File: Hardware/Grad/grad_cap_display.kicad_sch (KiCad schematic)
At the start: 11 parts, among them J101 Conn_01x06, J102 Conn_01x06, J103 Conn_01x06, J104 Conn_01x06, J105 Conn_01x06, J106 Conn_01x06, J107 Conn_01x06, J108 Conn_01x06, J109 Conn_01x06

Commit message: Schematic feels done now
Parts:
- J101, J102, J103, J104, J105, J106, J107, J108, J109: value Conn_01x06 -> 6-Pos 2.54mm Header; footprint (none) -> Connector_PinHeader_2.54mm:PinHeader_1x06_P2.54mm_Vertical
- R101, R102: footprint (none) -> New_Library:Worthington_R_0402
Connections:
- net RS485_B renamed FRAME_SYNC
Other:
- added sheet SAMD21 (SAMD21.kicad_sch)
- sheet ESP32 1 ports: added BACKLIGHT_PWM_IN, FRAME_SYNC_IN, SPI_CS_µSD, SPI_MISO_µSD, SPI_MOSI_µSD, SPI_SCK_µSD; removed FRAME_SYNC
- sheet ESP32 2 ports: added BACKLIGHT_PWM_IN, FRAME_SYNC_IN, SPI_CS_µSD, SPI_MISO_µSD, SPI_MOSI_µSD, SPI_SCK_µSD; removed FRAME_SYNC
- sheet ESP32 3 ports: added BACKLIGHT_PWM_IN, FRAME_SYNC_IN, SPI_CS_µSD, SPI_MISO_µSD, SPI_MOSI_µSD, SPI_SCK_µSD; removed FRAME_SYNC
- sheet ESP32 4 ports: added BACKLIGHT_PWM_IN, FRAME_SYNC_IN, SPI_CS_µSD, SPI_MISO_µSD, SPI_MOSI_µSD, SPI_SCK_µSD; removed FRAME_SYNC
- sheet ESP32 5 ports: added BACKLIGHT_PWM_IN, FRAME_SYNC_IN, SPI_CS_µSD, SPI_MISO_µSD, SPI_MOSI_µSD, SPI_SCK_µSD; removed FRAME_SYNC
- sheet ESP32 6 ports: added BACKLIGHT_PWM_IN, FRAME_SYNC_IN, SPI_CS_µSD, SPI_MISO_µSD, SPI_MOSI_µSD, SPI_SCK_µSD; removed FRAME_SYNC
- sheet ESP32 7 ports: added BACKLIGHT_PWM_IN, FRAME_SYNC_IN, SPI_CS_µSD, SPI_MISO_µSD, SPI_MOSI_µSD, SPI_SCK_µSD; removed FRAME_SYNC
- sheet ESP32 8 ports: added BACKLIGHT_PWM_IN, FRAME_SYNC_IN, SPI_CS_µSD, SPI_MISO_µSD, SPI_MOSI_µSD, SPI_SCK_µSD; removed FRAME_SYNC
- sheet ESP32 9 ports: added BACKLIGHT_PWM_IN, FRAME_SYNC_IN, SPI_CS_µSD, SPI_MISO_µSD, SPI_MOSI_µSD, SPI_SCK_µSD; removed FRAME_SYNC
- moved on the sheet: J101, J102, J103, J104, J105, J106, J107, J108, J109, R101, R102

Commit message: Prototype of PCB layout
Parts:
- removed J101, J102, J103, J104, J105, J106, J107, J108, J109: 6-Pos 2.54mm Header, Connector_PinHeader_2.54mm:PinHeader_1x06_P2.54mm_Vertical, symbol Connector_Generic:Conn_01x06
- removed R101, R102: 120, New_Library:Worthington_R_0402, symbol Device:R_Small_US
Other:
- removed sheet ESP32 2
- removed sheet ESP32 3
- removed sheet ESP32 4
- removed sheet ESP32 5
- removed sheet ESP32 6
- removed sheet ESP32 7
- removed sheet ESP32 8
- removed sheet ESP32 9

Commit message: More routing progress
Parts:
- added C101, C102, C103, C104, C107, C113, C116: 22uF, New_Library:Worthington_C_0603, symbol Device:C_Polarized_Small_US
- added C105, C106, C108, C109, C110, C111, C112, C114, C115, C401: 100nF, New_Library:Worthington_C_0402, symbol Device:C_Small_US
- added C217, C220, C221, C402: 100nF, Capacitor_SMD:C_0402_1005Metric, symbol Device:C_Small_US
- added C218, C219, C222, C223: 22uF, Capacitor_SMD:C_0603_1608Metric, symbol Device:C_Polarized_Small_US
- added D101, D102, D103, D104, D105, D206, D207, D208: RED, New_Library:Worthington_LED_0603, symbol Device:LED_Small
- added J101: Power In, Connector_JST:JST_PH_S2B-PH-K_1x02_P2.00mm_Horizontal, symbol Connector_Generic:Conn_01x02
- added J102: 6-Pos 2.54mm Header, Connector_PinHeader_2.54mm:PinHeader_1x06_P2.54mm_Vertical_SMD_Pin1Left, symbol Connector_Generic:Conn_01x06
- added J103: 2x8 2.54mm IDC Header, Connector_IDC:IDC-Header_2x06_P2.54mm_Vertical_SMD, symbol Connector_Generic:Conn_02x06_Odd_Even
- added J104: Amphenol 40-Pin FPC, New_Library:AMPHENOL_62684-402100ALF, symbol Connector_Generic:Conn_01x40
- added J207: SPI TestPoint, Connector_PinHeader_2.54mm:PinHeader_1x06_P2.54mm_Vertical_SMD_Pin1Right, symbol Connector_Generic:Conn_01x06
- added J208: RS485 TestPoint, Connector_PinHeader_2.54mm:PinHeader_1x05_P2.54mm_Vertical_SMD_Pin1Right, symbol Connector_Generic:Conn_01x05
- added J209: Extra TestPoint, Connector_PinHeader_2.54mm:PinHeader_1x05_P2.54mm_Vertical_SMD_Pin1Right, symbol Connector_Generic:Conn_01x05
- added J210: Micro_SD_Card, New_Library:CUI_MSD-4-A, symbol Connector:Micro_SD_Card
- added J211: Push Button Header, Connector_PinHeader_2.54mm:PinHeader_1x06_P2.54mm_Vertical_SMD_Pin1Right, symbol Connector_Generic:Conn_01x06
- added J401, J402, J403, J404: 01x30 Pads, Connector_PinSocket_2.54mm:PinSocket_1x30_P2.54mm_Vertical, symbol Connector_Generic:Conn_01x30
- added J405: LCD Power TestPoint, Connector_PinHeader_2.54mm:PinHeader_1x02_P2.54mm_Vertical_SMD_Pin1Right, symbol Connector_Generic:Conn_01x02
- added L101: 22uH, New_Library:CDRH5D28, symbol Device:L
- added R101, R209: 430, New_Library:Worthington_R_0402, symbol Device:R_Small_US
- added R102, R104, R105: 10, Resistor_SMD:R_1210_3225Metric, symbol Device:R_Small_US
- added R103, R204: 120, New_Library:Worthington_R_0402, symbol Device:R_Small_US
- added R207, R208: 1k, New_Library:Worthington_R_0402, symbol Device:R_Small_US
- added R401, R402, R403: 100, New_Library:Worthington_R_0402, symbol Device:R_Small_US
- added RN101, RN204: 10k, New_Library:RESCAXE80P320X160X70-8N, symbol Libraries:R_Network04_Split
- added RN102: 430, New_Library:RESCAXE80P320X160X70-8N, symbol Libraries:R_Network04_Split
- added RN203: 47k, New_Library:RESCAXE80P320X160X70-8N, symbol Libraries:R_Network04_Split
- added U101: LM66200DRLR, Package_TO_SOT_SMD:SOT-583-8, symbol Power_Management:LM66100DCK
- added U102: TLV75733PDRV, Package_SON:WSON-6-1EP_2x2mm_P0.65mm_EP1x1.6mm, symbol Regulator_Linear:TLV75733PDRV
- added U103: SN74LVC1G139, Package_SO:VSSOP-8_2.3x2mm_P0.5mm, symbol 74xGxx:74LVC1G139
- added U104: ESP32-S3-WROOM-1-N8R8, RF_Module:ESP32-S3-WROOM-1, symbol RF_Module:ESP32-S3-WROOM-1
- added U105, U209: TC7MBL3126CFT, Package_SO:TSSOP-14_4.4x5mm_P0.65mm, symbol Analog_Switch:CD4066BPW
- added U106: AP3019AKTTR, Package_TO_SOT_SMD:TSOT-23-6, symbol Driver_LED:AP3019AKTTR
- added U107, U210: THVD1400D, Package_SO:SOIC-8_3.9x4.9mm_P1.27mm, symbol Interface_UART:THVD1400D
- added U108: W25Q128JVP, Package_SON:WSON-8-1EP_6x5mm_P1.27mm_EP3.4x4.3mm, symbol Memory_Flash:W25Q128JVP
- added U211: AZ1117-5.0, Package_TO_SOT_SMD:SOT-89-3, symbol Regulator_Linear:AZ1117-5.0
- added U212: QTPy SAMD21, New_Library:Py_QT_SAMD21, symbol New_Library:QT_Py_SAMD21
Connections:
- new net: D102.2 (A), RN102.1 (4)
- new net: D105.2 (A), RN102.4
- new net: D104.2 (A), RN102.3
- new net: D206.2 (A), R207.1
- new net: D103.2 (A), RN102.2
- new net: J211.5 (Pin_5), RN204.3
- new net: J211.3 (Pin_3), RN204.6, RN204.7 (5)
- new net: J104.38 (LEDK), J104.39 (LEDK), R102.1, R104.1, R104.2, R105.1, R105.2, U106.3 (FB)
- new net: C114.1, C116.1, J104.40 (LEDA), J405.1 (Pin_1), U106.5 (V_{OUT})
- new net: D208.1 (K), R209.1
- new net: J404.1 (Pin_1), J404.10 (Pin_10), J404.11 (Pin_11), J404.12 (Pin_12), J404.13 (Pin_13), J404.14 (Pin_14), J404.15 (Pin_15), J404.16 (Pin_16), J404.17 (Pin_17), J404.18 (Pin_18), J404.19 (Pin_19), J404.2 (Pin_2), J404.20 (Pin_20), J404.21 (Pin_21), J404.22 (Pin_22), J404.23 (Pin_23), J404.24 (Pin_24), J404.3 (Pin_3), J404.4 (Pin_4), J404.7 (Pin_7), J404.8 (Pin_8), J404.9 (Pin_9)
- new net: L101.2, U106.1 (SW)
- new net: D207.1 (K), R208.1
- new net: J210.CD (CHIP_DETECT), R208.2
- new net: D101.1 (K), R101.1
- new net +3V3: C104.1, C105.1, C106.1, C107.1, C108.1, C109.1, C110.1, C111.1, C112.1, C401.1, D101.2 (A), J104.36 (VDD), RN101.1 (4), RN101.2, RN101.3, RN101.4, U102.1 (OUT), U103.8 (VCC), U104.2 (3V3), U105.14 (VCC), U107.8 (VCC), U108.8 (VCC)
- new net BACKLIGHT_PWM: J103.8 (Pin_8), J209.4 (Pin_4), U106.4 (CTRL), U212.6 (SCL)
- new net BATT_IN: C102.1, C113.1, C115.1, J101.1 (Pin_1), J401.25 (Pin_25), J401.26 (Pin_26), J401.5 (Pin_5), J401.6 (Pin_6), J402.25 (Pin_25), J402.26 (Pin_26), J402.5 (Pin_5), J402.6 (Pin_6), J403.25 (Pin_25), J403.26 (Pin_26), J403.5 (Pin_5), J403.6 (Pin_6), J404.25 (Pin_25), J404.26 (Pin_26), J404.5 (Pin_5), J404.6 (Pin_6), L101.1, U101.3 (VIN1), U106.6 (V_{IN})
- new net BUTTON_SENSE: J211.1 (Pin_1), RN204.1 (4), RN204.2, U212.4 (A3)
- new net ESP_CS0: U103.1 (A), U104.16 (IO46)
- new net ESP_CS1: U103.2 (B), U104.18 (IO10)
- new net ESP_CS_FLASH: RN101.7 (5), RN102.6, U103.6 (Y1), U108.1 (~{CS})
- new net ESP_CS_LCD: J104.30 (CS), RN101.8, RN102.5, U103.7 (Y0)
- new net ESP_CS_µSD: RN101.6, RN102.7 (5), U103.5 (Y2), U105.12 (A4)
- new net ESP_MISO: U104.26 (IO45), U105.3 (B1), U108.2 (DO/IO_{1})
- new net ESP_MOSI: R401.1, U104.12 (IO8), U105.5 (A2), U108.5 (DI/IO_{0})
- new net ESP_MOSI_T: J104.32 (SDA), R401.2
- new net ESP_PROG_EN: J102.2 (Pin_2), U104.3 (EN)
- new net ESP_PROG_IO0: J102.6 (Pin_6), U104.27 (IO0)
- new net ESP_PROG_PWR: C101.1, J102.1 (Pin_1), U101.6 (VIN2)
- new net ESP_PROG_RXD0: J102.5 (Pin_5), U104.36 (RXD0)
- new net ESP_PROG_TXD0: J102.4 (Pin_4), U104.37 (TXD0)
- new net ESP_SCK: R403.1, U104.17 (IO9), U105.9 (A3), U108.6 (CLK)
- new net ESP_SCK_T: J104.31 (SCK), R403.2
- new net ESP_µSD_BUS_CONNECT: RN101.5, RN102.8, U103.3 (Y3), U105.1 (1~{OE}), U105.10 (3~{OE}), U105.13 (4~{OE}), U105.4 (2~{OE})
- new net FRAME_SYNC: J103.10 (Pin_10), J209.3 (Pin_3), U104.39 (IO1), U212.3 (A2)
- new net GND: C101.2, C102.2, C103.2, C104.2, C105.2, C106.2, C107.2, C108.2, C109.2, C110.2, C111.2, C112.2, C113.2, C114.2, C115.2, C116.2, C217.2, C218.2, C219.2, C220.2, C221.2, C222.2, C223.2, C401.2, C402.2, D102.1 (K), D103.1 (K), D104.1 (K), D105.1 (K), D206.1 (K), J101.2 (Pin_2), J102.3 (Pin_3), J103.1 (Pin_1), J103.11 (Pin_11), J103.12 (Pin_12), J103.2 (Pin_2), J104.1 (GND), J104.37 (GND), J104.7 (GND), J104.S1 (M), J104.S2 (M), J207.1 (Pin_1), J208.1 (Pin_1), J208.5 (Pin_5), J209.1 (Pin_1), J209.5 (Pin_5), J210.6 (VSS), J210.9 (SHIELD), J211.2 (Pin_2), J211.4 (Pin_4), J211.6 (Pin_6), J401.1 (Pin_1), J401.10 (Pin_10), J401.11 (Pin_11), J401.12 (Pin_12), J401.13 (Pin_13), J401.14 (Pin_14), J401.15 (Pin_15), J401.16 (Pin_16), J401.17 (Pin_17), J401.18 (Pin_18), J401.19 (Pin_19), J401.2 (Pin_2), J401.20 (Pin_20), J401.21 (Pin_21), J401.22 (Pin_22), J401.23 (Pin_23), J401.24 (Pin_24), J401.27 (Pin_27), J401.28 (Pin_28), J401.29 (Pin_29), J401.3 (Pin_3), J401.30 (Pin_30), J401.4 (Pin_4), J401.7 (Pin_7), J401.8 (Pin_8), J401.9 (Pin_9), J402.1 (Pin_1), J402.10 (Pin_10), J402.11 (Pin_11), J402.12 (Pin_12), J402.13 (Pin_13), J402.14 (Pin_14), J402.15 (Pin_15), J402.16 (Pin_16), J402.17 (Pin_17), J402.18 (Pin_18), J402.19 (Pin_19), J402.2 (Pin_2), J402.20 (Pin_20), J402.21 (Pin_21), J402.22 (Pin_22), J402.23 (Pin_23), J402.24 (Pin_24), J402.27 (Pin_27), J402.28 (Pin_28), J402.29 (Pin_29), J402.3 (Pin_3), J402.30 (Pin_30), J402.4 (Pin_4), J402.7 (Pin_7), J402.8 (Pin_8), J402.9 (Pin_9), J403.1 (Pin_1), J403.10 (Pin_10), J403.11 (Pin_11), J403.12 (Pin_12), J403.13 (Pin_13), J403.14 (Pin_14), J403.15 (Pin_15), J403.16 (Pin_16), J403.17 (Pin_17), J403.18 (Pin_18), J403.19 (Pin_19), J403.2 (Pin_2), J403.20 (Pin_20), J403.21 (Pin_21), J403.22 (Pin_22), J403.23 (Pin_23), J403.24 (Pin_24), J403.27 (Pin_27), J403.28 (Pin_28), J403.29 (Pin_29), J403.3 (Pin_3), J403.30 (Pin_30), J403.4 (Pin_4), J403.7 (Pin_7), J403.8 (Pin_8), J403.9 (Pin_9), J404.27 (Pin_27), J404.28 (Pin_28), J404.29 (Pin_29), J404.30 (Pin_30), J405.2 (Pin_2), R101.2, R102.2, R209.2, U101.1 (GND), U101.4 (~{ON}), U101.5 (GND), U102.2 (NC), U102.3 (GND), U102.5 (NC), U102.7 (GND), U103.4 (GND), U104.1 (GND), U104.40 (GND), U104.41 (GND), U105.7 (GND), U106.2 (GND), U107.5 (GND), U108.4 (GND), U209.7 (GND), U210.5 (GND), U211.1 (GND), U212.13 (GND)
- new net LCD_RGB_DB0: J104.25 (DB0), U104.38 (IO2)
- new net LCD_RGB_DB1: J104.24 (DB1), U104.4 (IO4)
- new net LCD_RGB_DB10: J104.15 (DB10), U104.11 (IO18)
- new net LCD_RGB_DB11: J104.14 (DB11), U104.13 (USB_D-)
- new net LCD_RGB_DB12: J104.13 (DB12), U104.14 (USB_D+)
- new net LCD_RGB_DB13: J104.12 (DB13), U104.35 (IO42)
- new net LCD_RGB_DB14: J104.11 (DB14), U104.24 (IO47)
- new net LCD_RGB_DB15: J104.10 (DB15), U104.25 (IO48)
- new net LCD_RGB_DB16: J104.9 (DB16)
- new net LCD_RGB_DB17: J104.8 (DB17)
- new net LCD_RGB_DB2: J104.23 (DB2), U104.5 (IO5)
- new net LCD_RGB_DB3: J104.22 (DB3), U104.6 (IO6)
- new net LCD_RGB_DB4: J104.21 (DB4), U104.7 (IO7)
- new net LCD_RGB_DB5: J104.20 (DB5), U104.21 (IO13)
- new net LCD_RGB_DB6: J104.19 (DB6), U104.22 (IO14)
- new net LCD_RGB_DB7: J104.18 (DB7), U104.8 (IO15)
- new net LCD_RGB_DB8: J104.17 (DB8), U104.9 (IO16)
- new net LCD_RGB_DB9: J104.16 (DB9), U104.10 (IO17)
- new net LCD_RGB_DE: J104.28 (DE), U104.32 (IO39)
- new net LCD_RGB_HSYNC: J104.26 (HS), U104.34 (IO41)
- new net LCD_RGB_PCLK: J104.29 (PCLK), U104.31 (IO38)
- new net LCD_RGB_VSYNC: J104.27 (VS), U104.33 (IO40)
- new net PWR_IN: C103.1, C218.1, U101.2 (VOUT), U101.7 (VOUT), U102.4 (EN), U102.6 (IN), U211.3 (VI)
- new net RS485_A: J103.4 (Pin_4), R103.1, R204.1, U107.6 (A), U210.6 (A)
- new net RS485_B: J103.6 (Pin_6), R103.2, R204.2, U107.7 (B), U210.7 (B)
- new net SAMD21_3V3: C217.1, C221.1, C222.1, C223.1, C402.1, D207.2 (A), D208.2 (A), J210.4 (VDD), RN203.1 (4), RN203.2, RN203.3, RN203.4, RN204.8, U209.14 (VCC), U210.8 (VCC), U212.12 (3V)
- new net SAMD21_5V: C219.1, C220.1, R207.2, U211.2 (VO), U212.14 (5V)
- new net SAMD_CS_µSD: J207.3 (Pin_3), U209.12 (A4), U212.2 (A1)
- new net SAMD_MISO: J207.5 (Pin_5), U209.3 (B1), U212.10 (MI)
- new net SAMD_MOSI: J207.4 (Pin_4), U209.5 (A2), U212.11 (MO)
- new net SAMD_SCK: J207.6 (Pin_6), U209.9 (A3), U212.9 (SCK)
- new net SAMD_UART-RS485_DE: J208.2 (Pin_2), U210.2 (~{RE}), U210.3 (DE), U212.5 (SDA)
- new net SAMD_UART-RS485_RX: J208.4 (Pin_4), U210.1 (RO), U212.8 (RX)
- new net SAMD_UART-RS485_TX: J208.3 (Pin_3), U210.4 (DI), U212.7 (TX)
- new net SAMD_µSD_BUS_CONNECT: J207.2 (Pin_2), U209.1 (1~{OE}), U209.10 (3~{OE}), U209.13 (4~{OE}), U209.4 (2~{OE}), U212.1 (A0)
- new net STRAP_GPIO3: U104.15 (IO3)
- new net UART-RS485_RX: U104.20 (IO12), U107.1 (RO)
- new net UART-RS485_TX: U104.19 (IO11), U107.4 (DI)
- new net UART_RS485_DE: U104.23 (IO21), U107.2 (~{RE}), U107.3 (DE)
- new net µSD_SPI_CS: J103.3 (Pin_3), J210.2 (DAT3/CD), RN203.5, U105.11 (B4), U209.11 (B4)
- new net µSD_SPI_MISO: J103.9 (Pin_9), J210.7 (DAT0), R402.2, RN203.6, U105.2 (A1)
- new net µSD_SPI_MISO_T: R402.1, U209.2 (A1)
- new net µSD_SPI_MOSI: J103.7 (Pin_7), J210.3 (CMD), RN203.7 (5), U105.6 (B2), U209.6 (B2)
- new net µSD_SPI_SCK: J103.5 (Pin_5), J210.5 (CLK), RN203.8, U105.8 (B3), U209.8 (B3)
- no-connect marks 0 -> 1
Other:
- removed sheet ESP32 1
- removed sheet SAMD21
- note added: "Italics denote bootstrapping pins which go to weird states upon ESP32 reset. Be aware that these might be weird to get configured in software."
- note added: "Populate 120R Resistor If Last Panel In Chain"
- note added: "QTPy SAMD21 has +5V -> +3V3 Regulator Onboard "3V" Pin is the output from this regulator"

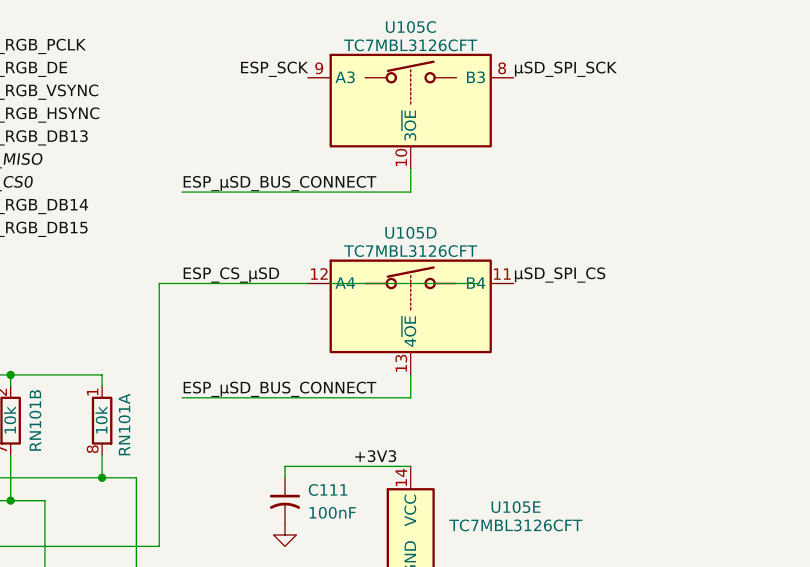
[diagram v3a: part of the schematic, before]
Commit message: Small tweaks
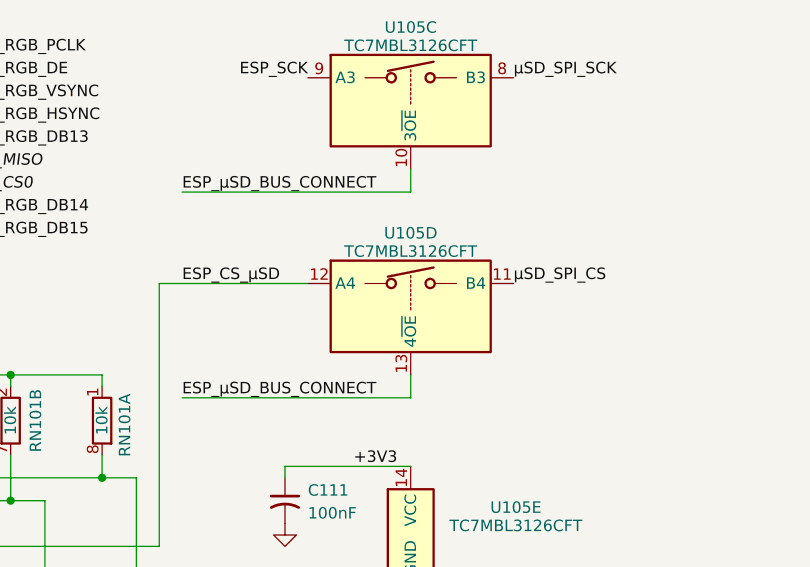
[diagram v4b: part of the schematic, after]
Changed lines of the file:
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@@
-	(wire
-		(pts
-			(xy 242.57 90.17) (xy 259.08 90.17)
-		)
-		(stroke
-			(width 0)
-			(type default)
-		)
-	)
 	(wire
 		(pts
